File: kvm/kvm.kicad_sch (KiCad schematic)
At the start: 61 parts, among them J1 USB4110-GF-A, J2 USB4110-GF-A, J3 USB_A_Stacked, J4 USB_A_Stacked, Q1 Q_PMOS_GSD, SW1 SW_DPDT_x2, U1 SRV05-4, U2 LTC4412xS6, U3 FSUSB42MUX, U4 GL850G, U5 SRV05-4, U6 SRV05-4, Y1 Crystal

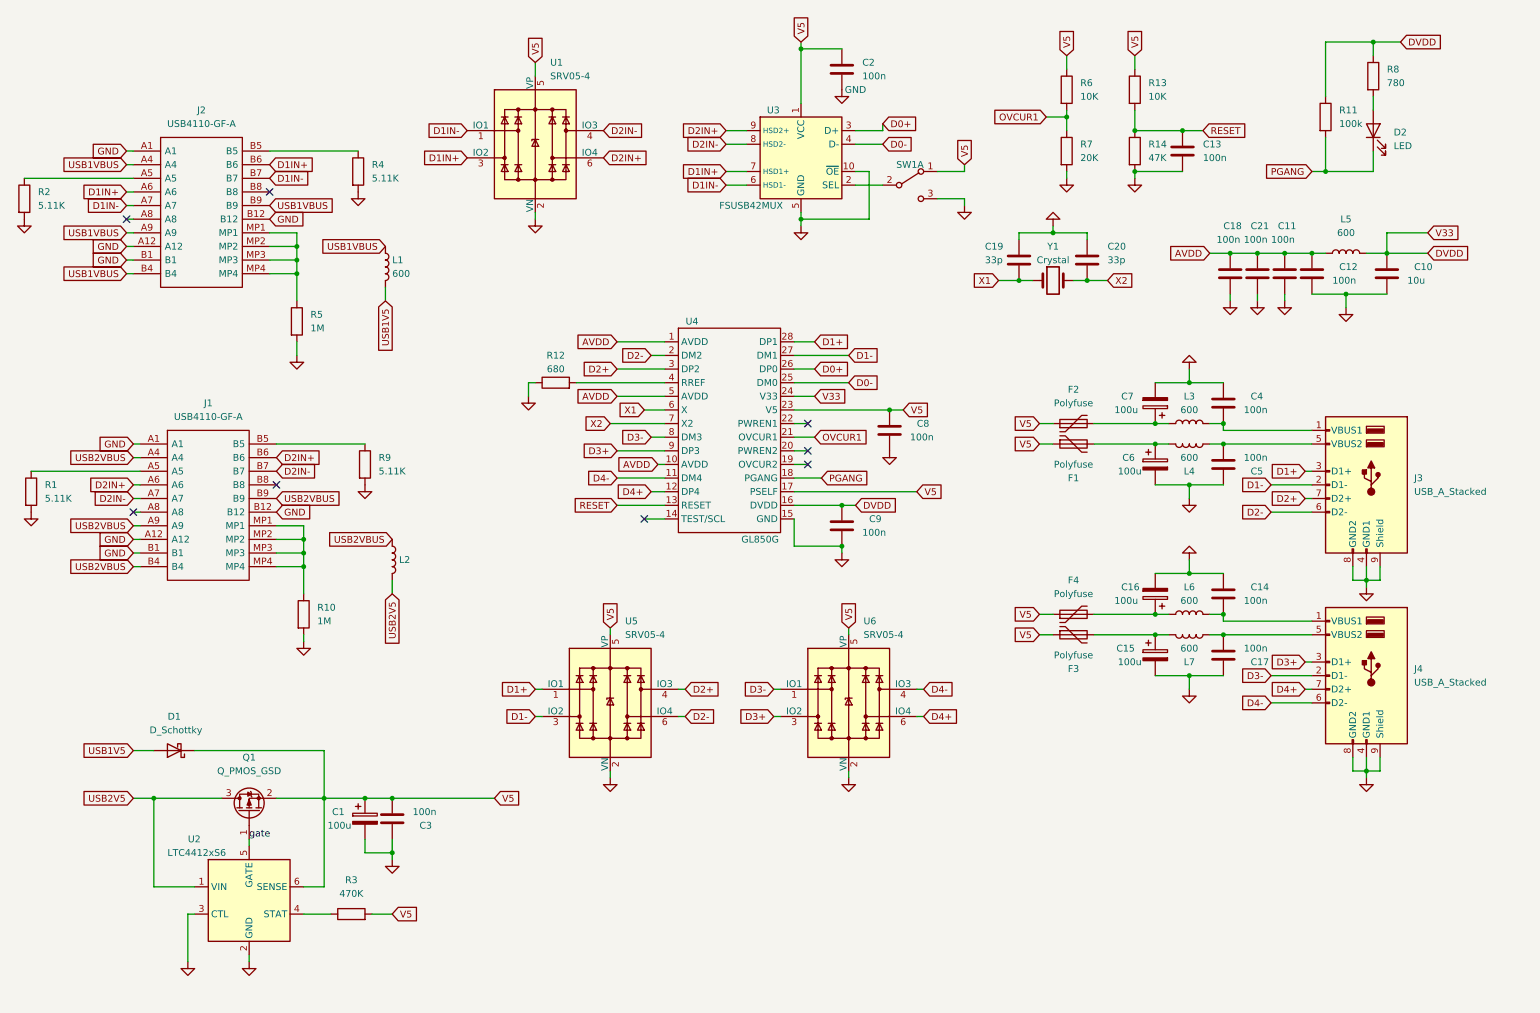
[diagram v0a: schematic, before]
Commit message: added gerber files
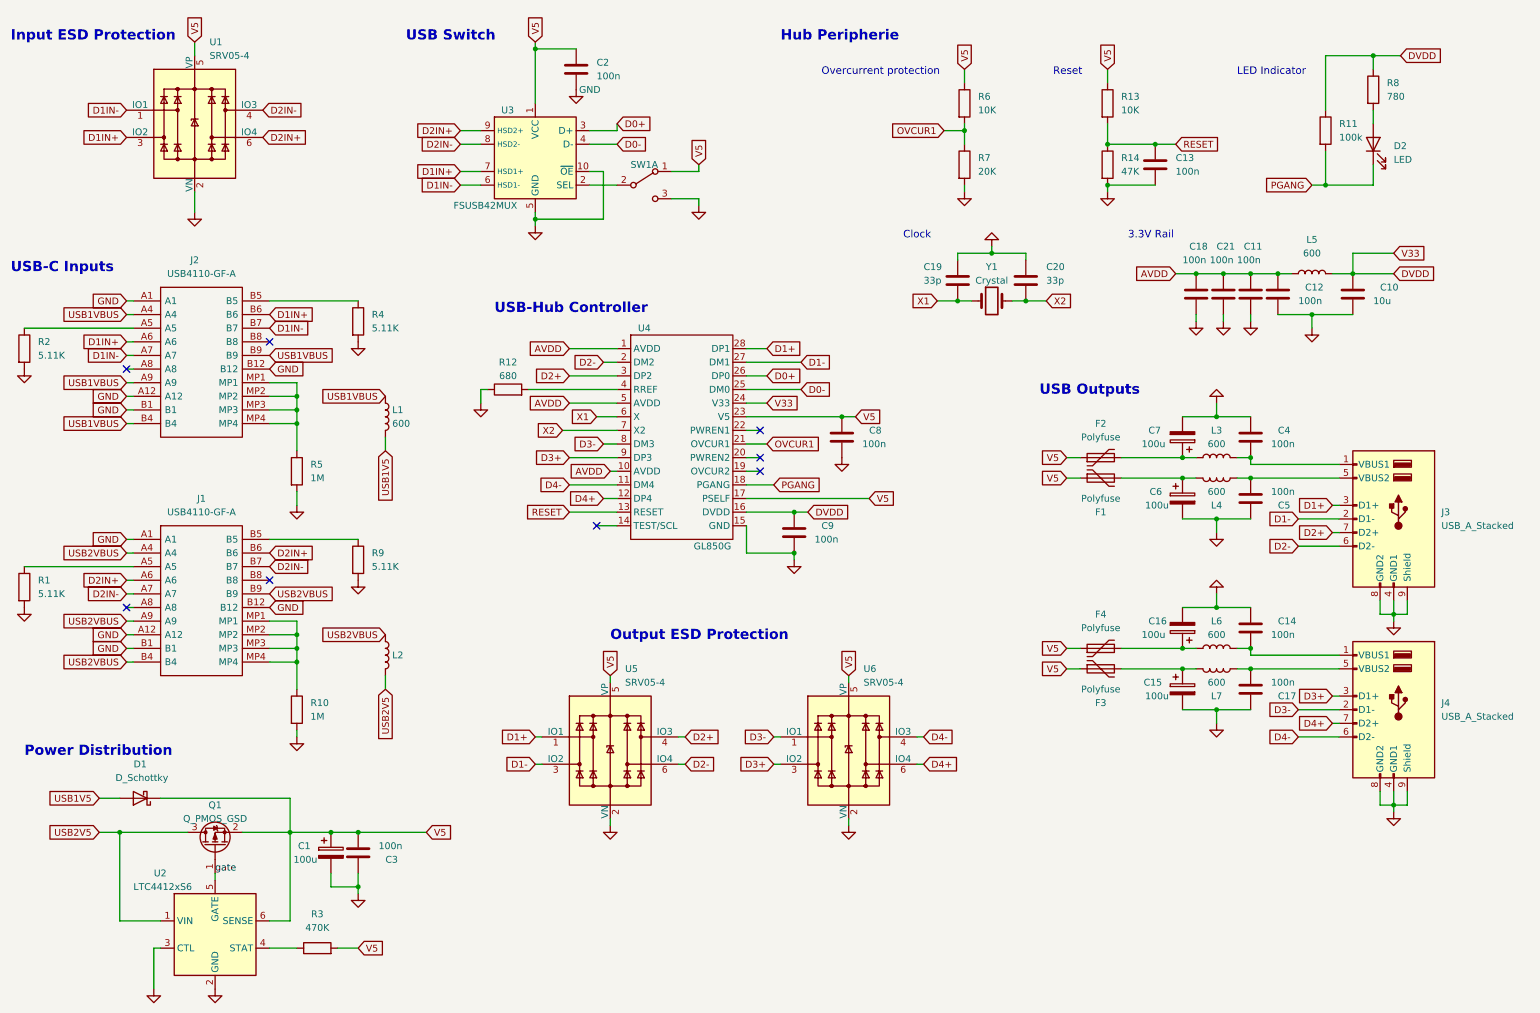
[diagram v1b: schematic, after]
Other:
- note added: "3.3V Rail"
- note added: "Clock"
- note added: "Hub Peripherie"
- note added: "Input ESD Protection"
- note added: "LED Indicator"
- note added: "Output ESD Protection"
- note added: "Overcurrent protection"
- note added: "Power Distribution"
- note added: "Reset"
- note added: "USB Outputs"
- note added: "USB Switch"
- note added: "USB-C Inputs"
- note added: "USB-Hub Controller"
- moved on the sheet: C1, C10, C11, C12, C13, C14, C15, C16, C17, C18, C19, C2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

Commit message: added buy links
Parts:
- C10: MouserLink (none) -> https://www.mouser.at/ProductDetail/Taiyo-Yuden/LMK212ABJ10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
- C11, C12, C14, C17, C18, C21, C4, C5: MouserLink (none) -> https://www.mouser.at/ProductDetail/TDK/C0603X5R1E104K030BB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
- C15, C16, C6, C7: MouserLink (none) -> https://www.mouser.at/ProductDetail/Panasonic/EEU-FR1C101?q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
- C20: MouserLink (none) -> https://www.mouser.at/ProductDetail/KYOCERA-AVX/06033A330FA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
- D1: MouserLink (none) -> https://www.mouser.at/ProductDetail/ROHM-Semiconductor/RB16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
- D2: MouserLink (none) -> https://www.mouser.at/ProductDetail/Kingbright/APTD2012LSUR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
- F1, F2, F3, F4: MouserLink (none) -> https://www.mouser.at/ProductDetail/Littelfuse/1206L050YR?q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
- J1, J2: MouserLink (none) -> https://www.mouser.at/ProductDetail/GCT/USB4110-GF-A?qs=KUo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
- J3, J4: MouserLink (none) -> https://www.mouser.at/ProductDetail/Wurth-Elektronik/614008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
- Q1: MouserLink (none) -> https://www.mouser.at/ProductDetail/Toshiba/SSM3J372RLXHF?q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
- U1, U5, U6: MouserLink (none) -> https://www.mouser.at/ProductDetail/Littelfuse/SRV05-4HTG-D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
- U2: MouserLink (none) -> https://www.mouser.at/ProductDetail/Analog-Devices/LTC4412I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
- U3: MouserLink (none) -> https://www.mouser.at/ProductDetail/onsemi-Fairchild/FSUSB4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
- U4: MouserLink (none) -> https://www.mouser.at/ProductDetail/Olimex-Ltd/GL850G?qs=do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
- Y1: MouserLink (none) -> https://www.mouser.at/ProductDetail/ECS/ECS-120-18-4X-CKM?q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
